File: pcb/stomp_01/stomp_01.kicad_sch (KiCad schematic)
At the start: 15 parts, among them J1 Conn_01x18_Pin, J10 Conn_01x18_Pin, J2 Conn_01x18_Pin, J3 Conn_01x18_Pin, J4 Conn_01x18_Pin, J5 Conn_01x18_Pin, J6 Conn_01x18_Pin, J7 Conn_01x18_Pin, J8 Conn_01x18_Pin, J9 Conn_01x18_Pin, U1 Teensy4.1

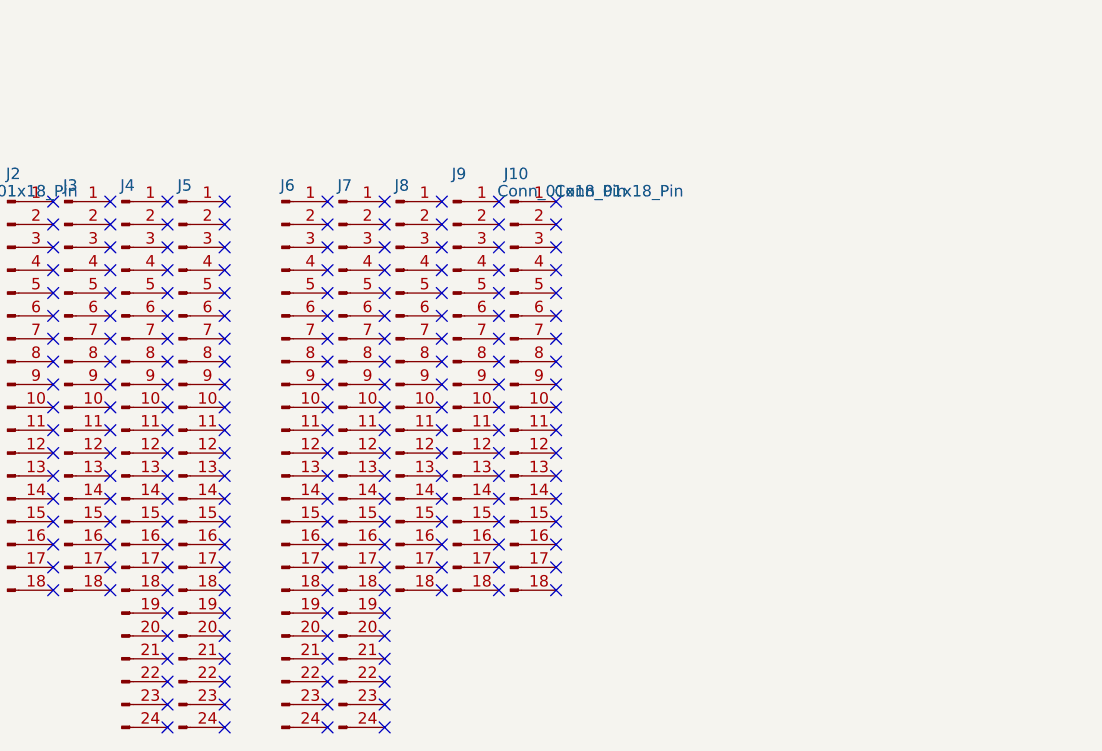
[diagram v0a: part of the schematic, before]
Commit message: pre routing
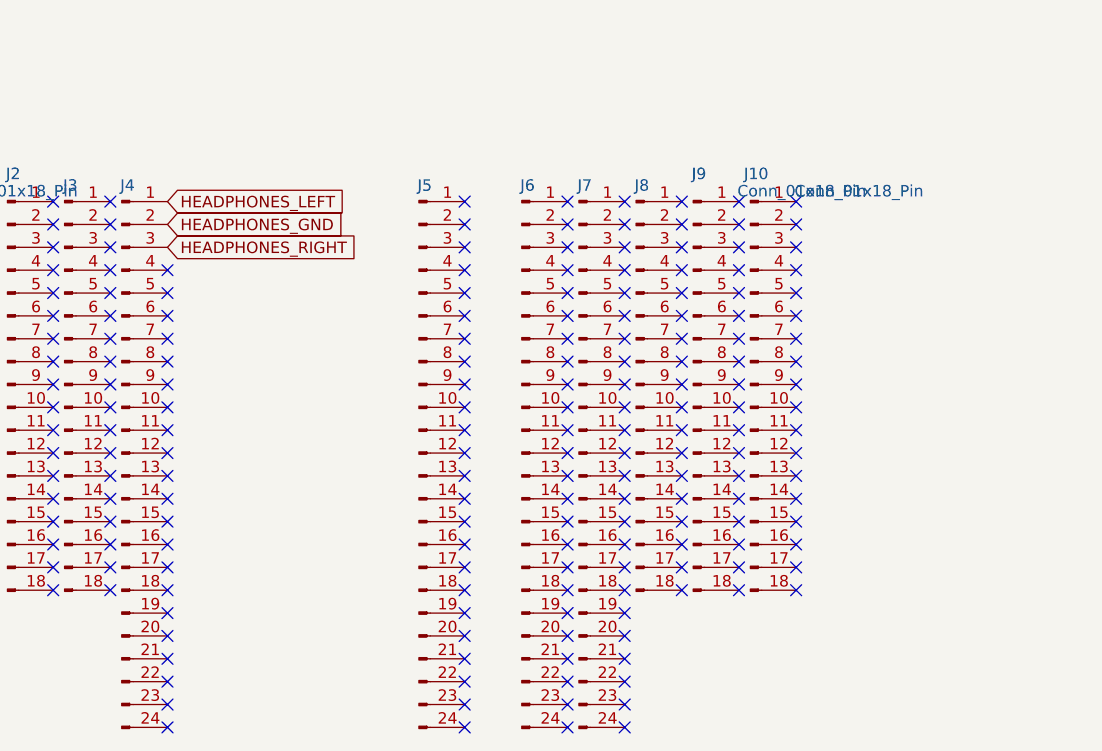
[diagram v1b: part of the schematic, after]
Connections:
- net HEADPHONES_LEFT: now reaches J4.1 (Pin_1)
- net HEADPHONES_GND: now reaches J4.2 (Pin_2)
- net HEADPHONES_RIGHT: now reaches J4.3 (Pin_3)
- no-connect marks 222 -> 219
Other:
- moved on the sheet: J10, J5, J6, J7, J8, J9
